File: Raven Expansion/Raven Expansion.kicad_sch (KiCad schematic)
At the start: 5 parts, among them J1 Conn_01x06_Pin, J2 Screw_Terminal_01x06, J3 Screw_Terminal_01x06

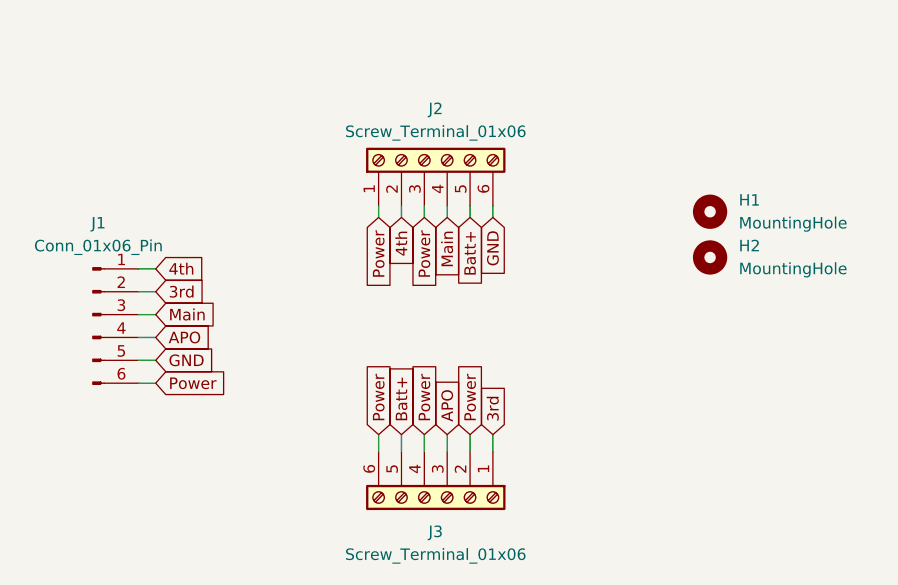
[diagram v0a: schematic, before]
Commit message: Ahhhhh
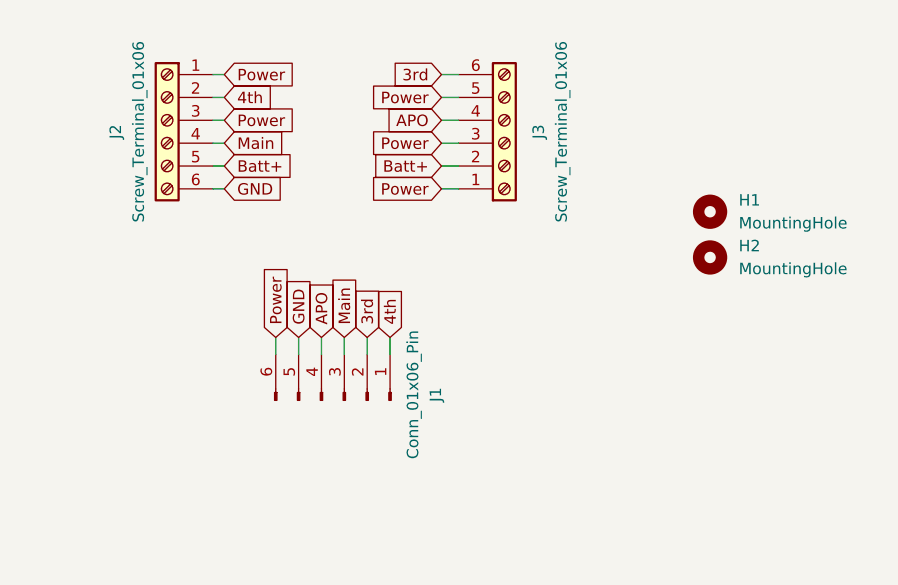
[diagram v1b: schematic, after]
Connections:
- net 3rd: now also J3.6 (Pin_6); no longer J3.1 (Pin_1)
- net APO: now also J3.4 (Pin_4); no longer J3.3 (Pin_3)
- net Batt+: now also J3.2 (Pin_2); no longer J3.5 (Pin_5)
- net Power: now also J3.1 (Pin_1), J3.3 (Pin_3), J3.5 (Pin_5); no longer J3.2 (Pin_2), J3.4 (Pin_4), J3.6 (Pin_6)
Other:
- moved on the sheet: J1, J2, J3
